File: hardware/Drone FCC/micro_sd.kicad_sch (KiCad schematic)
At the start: 9 parts, among them J701 DM3AT-SF-PEJM5

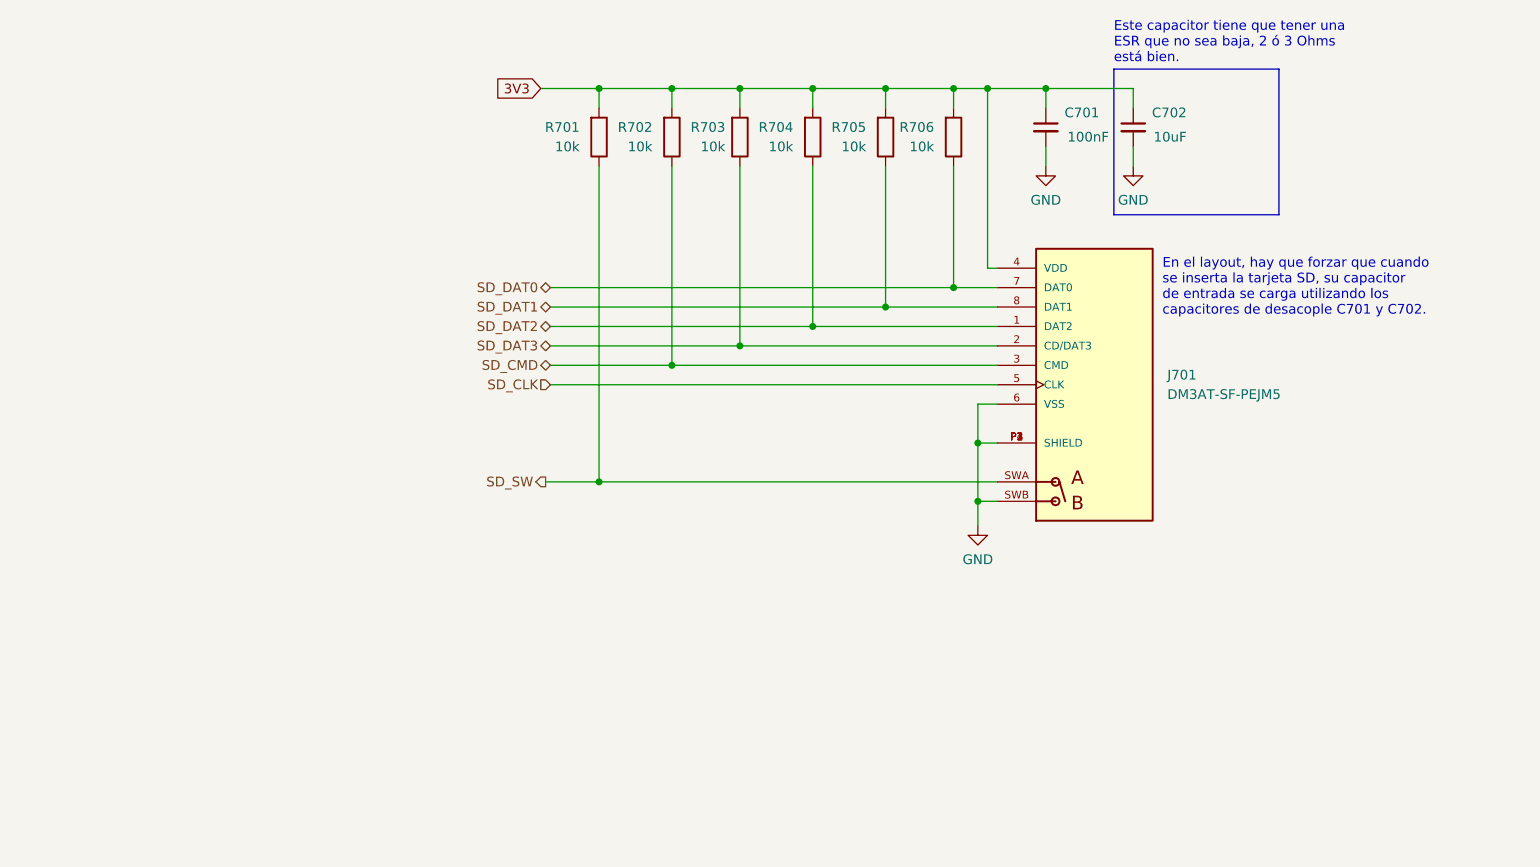
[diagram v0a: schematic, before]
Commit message: finish SD routing
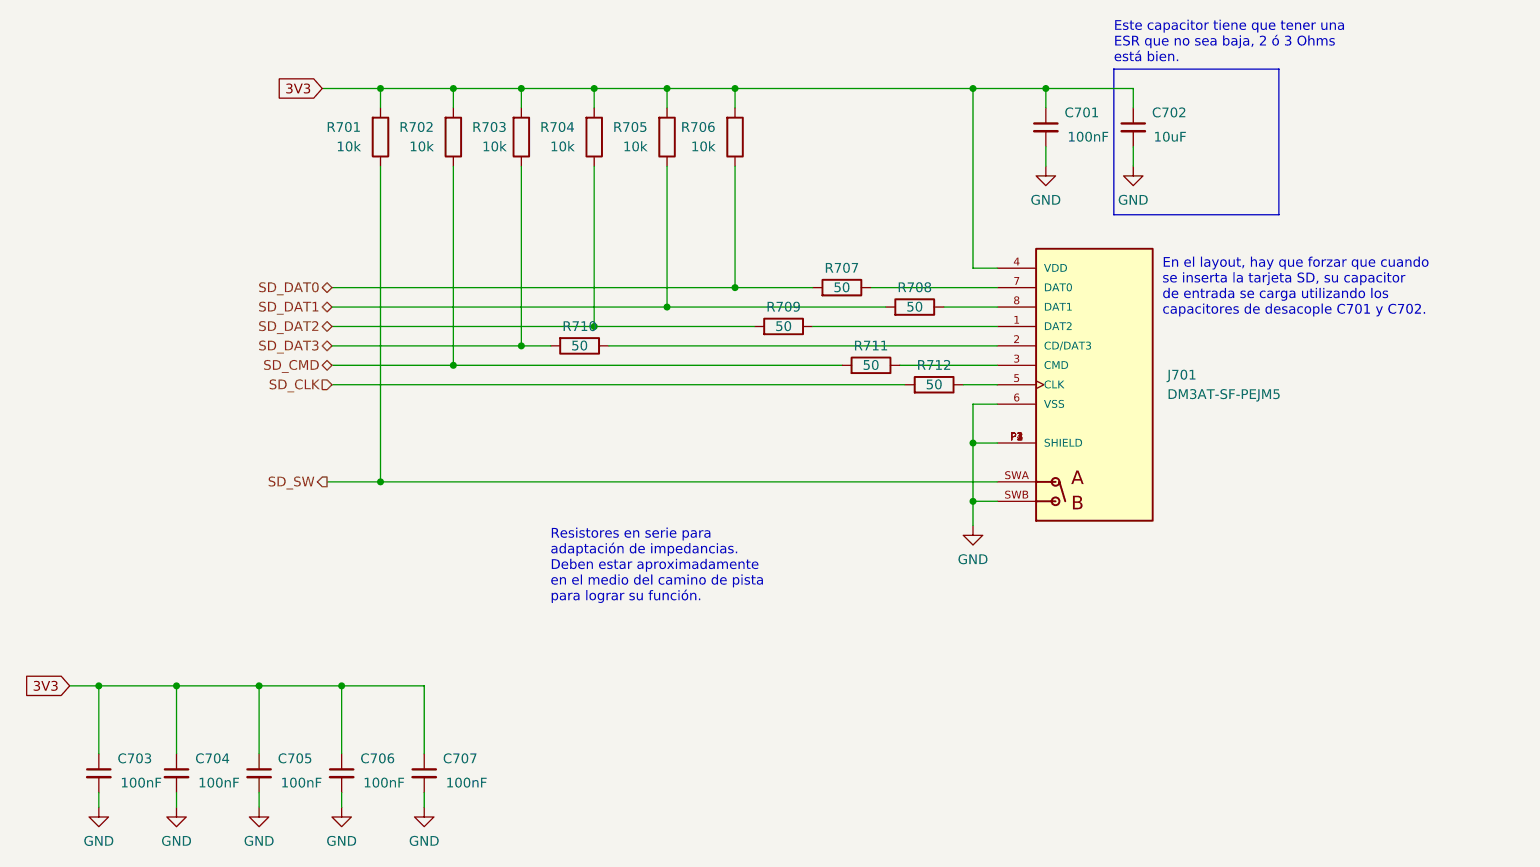
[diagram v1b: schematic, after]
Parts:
- added C703, C704, C705, C706, C707: 100nF, Capacitor_SMD:C_0402_1005Metric_Pad0.74x0.62mm_HandSolder, symbol Device:C_Small
- added R707, R708, R709, R710, R711, R712: 50, Resistor_SMD:R_0402_1005Metric_Pad0.72x0.64mm_HandSolder, symbol Device:R
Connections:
- net 3V3: now also C703.1, C704.1, C705.1, C706.1, C707.1
- net GND: now also C703.2, C704.2, C705.2, C706.2, C707.2
- net SD_CLK: now also R712.2; no longer J701.5 (CLK)
- net SD_CMD: now also R711.2; no longer J701.3 (CMD)
- net SD_DAT0: now also R707.2; no longer J701.7 (DAT0)
- net SD_DAT1: now also R708.2; no longer J701.8 (DAT1)
- net SD_DAT2: now also R709.2; no longer J701.1 (DAT2)
- net SD_DAT3: now also R710.2; no longer J701.2 (CD/DAT3)
- new net: J701.7 (DAT0), R707.1
- new net: J701.1 (DAT2), R709.1
- new net: J701.2 (CD/DAT3), R710.1
- new net: J701.3 (CMD), R711.1
- new net: J701.5 (CLK), R712.1
- new net: J701.8 (DAT1), R708.1
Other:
- note added: "Resistores en serie para adaptación de impedancias. Deben estar aproximadamente en el medio del camino de pista para lograr su función."
- moved on the sheet: R701, R702, R703, R704, R705, R706
